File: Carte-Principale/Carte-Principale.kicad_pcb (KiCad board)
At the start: 2 copper layers, 154.6 x 118.1 mm, 115 parts, among them J1 Moteur_Gauche, J10 GPIO, J11 I2C2, J12 GPIO, J13 Encodeur_G, J14 I2C_Sensors, J15 AX12, J16 GPIO, J17 SMD_Conn, J18 PCA9685, J19 GPIO, J2 GND, J3 12VA, J4 5V, J5 Moteur_Droit, J6 UART_Debug, J7 UART, J8 Encodeur_D, J9 SPI3, Q2 BSS138, Q3 BSS138, Q4 BSS138, Q5 BSS138, SW1 Rouge, SW2 Bleu, SW3 Jaune, SW4 Vert, U2 NUCLEOH723ZG, U3 AM26LV32xD, U4 74LVC1G3157, U5 74LVC1G3157, U6 74LVC1G3157, U7 74LVC1G3157

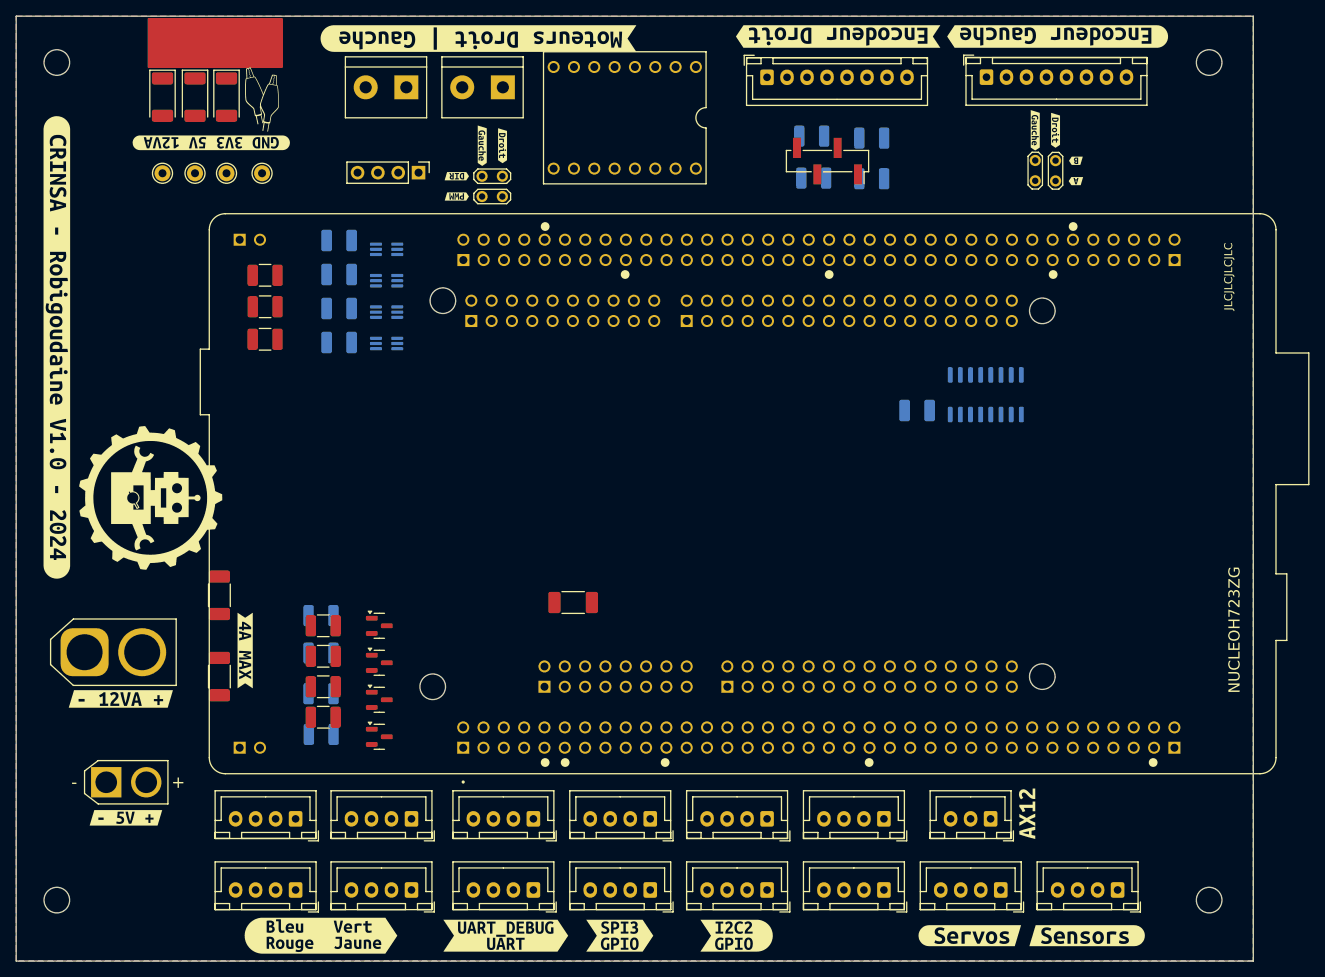
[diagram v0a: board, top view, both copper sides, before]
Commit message: FInal
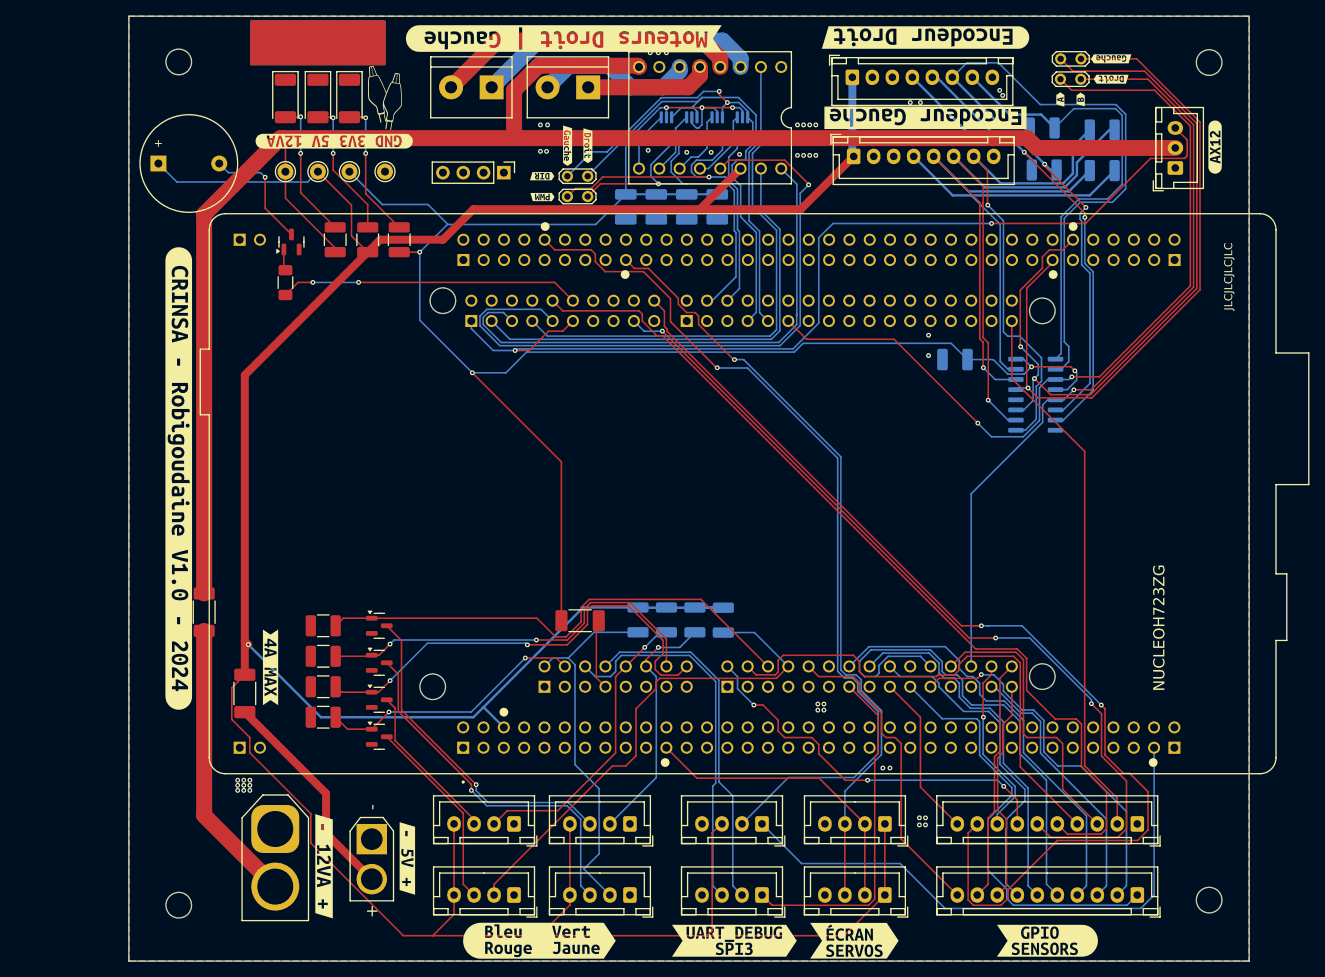
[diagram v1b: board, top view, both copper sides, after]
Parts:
- removed J11: I2C2, Connector_JST:JST_XH_B4B-XH-A_1x04_P2.50mm_Vertical
- removed J12, J16, J19: GPIO, Connector_JST:JST_XH_B4B-XH-A_1x04_P2.50mm_Vertical
- removed J14: I2C_Sensors, Connector_JST:JST_XH_B4B-XH-A_1x04_P2.50mm_Vertical
- removed J17: SMD_Conn, Connector_PinHeader_2.54mm:PinHeader_1x04_P2.54mm_Vertical_SMD_Pin1Right
- removed kibuzzard-11: G***, kibuzzard-66C08EB4
- removed kibuzzard-12: G***, kibuzzard-66C48662
- removed kibuzzard-13: G***, kibuzzard-66C46925
- removed kibuzzard-14: G***, kibuzzard-66C08BB8
- removed kibuzzard-26: G***, kibuzzard-66C091C7
- removed kibuzzard-31: G***, kibuzzard-66C09378
- removed kibuzzard-32: G***, kibuzzard-66C60E06
- removed kibuzzard-33: G***, kibuzzard-66C60E22
- removed kibuzzard-36: G***, kibuzzard-66C09018
- removed kibuzzard-66E9AA77: G***, kibuzzard-66E9AA77
- removed kibuzzard-66F082DD: G***, kibuzzard-66F082DD
- removed kibuzzard-66FEA7C0: G***, kibuzzard-66FEA7C0
- removed kibuzzard-66FEA7DC: G***, kibuzzard-66FEA7DC
- removed kibuzzard-66FEA7EE: G***, kibuzzard-66FEA7EE
- removed kibuzzard-66FEA7FA: G***, kibuzzard-66FEA7FA
- removed kibuzzard-9: G***, kibuzzard-66C092F4
- added BZ1: Buzzer, Buzzer_Beeper:Buzzer_12x9.5RM7.6, F.Cu at (73.7, 47.6)
- added J21: I2C Screen, Connector_JST:JST_XH_B4B-XH-A_1x04_P2.50mm_Vertical, F.Cu at (164.5, 130.2)
- added Q1: BC817, Package_TO_SOT_SMD:SOT-23, F.Cu at (90.3, 57.4)
- added R2: R, Resistor_SMD:R_1206_3216Metric_Pad1.30x1.75mm_HandSolder, F.Cu at (89.5, 62.5)
- added kibuzzard-67547681: G***, kibuzzard-67547681, F.Cu at (145.7, 144.8)
- added kibuzzard-67548783: G***, kibuzzard-67548783, F.Cu at (184.8, 144.8)
- added kibuzzard-67548923: G***, kibuzzard-67548923, F.Cu at (205.7, 45.6)
- added kibuzzard-6754898D: G***, kibuzzard-6754898D, B.Cu at (160.7, 134.6)
- added kibuzzard-675489B9: G***, kibuzzard-675489B9, B.Cu at (160.6, 142.6)
- added kibuzzard-675489F8: G***, kibuzzard-675489F8, B.Cu at (184.8, 143.5)
- added kibuzzard-67548A22: G***, kibuzzard-67548A22, B.Cu at (184.8, 134.0)
- added kibuzzard-67548BCB: G***, kibuzzard-67548BCB, F.Cu at (160.7, 144.8)
- added kibuzzard-6757392E: G***, kibuzzard-6757392E, F.Cu at (121.7, 51.8)
- added kibuzzard-67573990: G***, kibuzzard-67573990, F.Cu at (169.5, 31.9)
- added kibuzzard-675739BC: G***, kibuzzard-675739BC, F.Cu at (169.5, 41.9)
- G1: moved to B.Cu
- J10: value GPIO -> Sensors; footprint Connector_JST:JST_XH_B4B-XH-A_1x04_P2.50mm_Vertical -> Connector_JST:JST_XH_B10B-XH-A_1x10_P2.50mm_Vertical
- J7: value UART -> GPIO; footprint Connector_JST:JST_XH_B4B-XH-A_1x04_P2.50mm_Vertical -> Connector_JST:JST_XH_B10B-XH-A_1x10_P2.50mm_Vertical
- moved kibuzzard-27 90.4 mm to (197.5, 45.8), turned to 0 degrees
- moved J15 84.6 mm to (200.8, 48.2), turned to 90 degrees
- moved J7 75.9 mm to (196.0, 130.2)
- moved G1 74.0 mm to (146.7, 88.9)
- moved J10 60.9 mm to (196.0, 139.1)
- moved R34 52.3 mm to (144.3, 104.7), turned to 90 degrees
- moved U6 52.0 mm to (146.7, 43.2), turned to 90 degrees
- moved C6 50.2 mm to (143.5, 53.0), turned to 90 degrees
- moved U7 47.3 mm to (143.5, 43.2), turned to 90 degrees
- moved R33 46.7 mm to (140.7, 104.7), turned to 90 degrees
- moved C5 45.3 mm to (139.7, 53.0), turned to 90 degrees
- moved R31 44.2 mm to (137.2, 104.7), turned to 90 degrees
- moved U5 42.7 mm to (140.3, 43.2), turned to 90 degrees
- moved C4 40.5 mm to (135.9, 53.0), turned to 90 degrees
- moved R32 39.8 mm to (133.6, 104.7), turned to 90 degrees
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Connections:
- J10 pad 1: /PF8 -> /I2C2_SCL
- J10 pad 2: /PG1 -> /I2C2_SDA
- J10 pad 3: /PG0 -> /PD1
- J10 pad 4: /PD1 -> /PE2
- J7 pad 1: /PC7 -> GND
- J7 pad 2: /PC6 -> /PE0
- J7 pad 3: +5V -> /PF8
- J7 pad 4: GND -> /PD6
- U2 pad CN10_11: /PF6 -> /Encodeur_Droit_A
- U2 pad CN11_11: /Encodeur_Droit_B -> unconnected-(U2A-PF7-PadCN11_11)
- U2 pad CN11_41: /AX12_RX -> unconnected-(U2A-PD5-PadCN11_41)
- U2 pad CN11_6: unconnected-(U2A-5V_EXT-PadCN11_6) -> +5V
- U2 pad CN11_9: /Encodeur_Droit_A -> unconnected-(U2A-PF6-PadCN11_9)
- U2 pad CN12_37: /AX12_RX -> unconnected-(U2B-PA3-PadCN12_37)
- U2 pad CN7_1: /PC6 -> /AX12_RX
- U2 pad CN7_11: /PC7 -> /AX12_RX
- U2 pad CN9_26: /PF7 -> /Encodeur_Droit_B
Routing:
- net +5V: track 0.00 -> 418.8 mm, vias 0 -> 1
- net +3.3V: track 0.00 -> 240.8 mm, vias 0 -> 7
- net +12VA: track 0.00 -> 213.3 mm
- net /PF3: track 0.00 -> 134.4 mm, vias 0 -> 2
- net /AX12_RX: track 0.00 -> 120.8 mm, vias 0 -> 2
- net /PA5: track 0.00 -> 112.2 mm
- net /DEBUG_TX: track 0.00 -> 110.5 mm, vias 0 -> 1
- net /PA4: track 0.00 -> 107.0 mm, vias 0 -> 3
- net /Encodeur_Droit_A: track 0.00 -> 105.1 mm, vias 0 -> 2
- net /Encodeur_Droit_B: track 0.00 -> 98.1 mm, vias 0 -> 1
- net /I2C1_SCL: track 0.00 -> 97.7 mm, vias 0 -> 1
- net /Encodeur_Gauche_A: track 0.00 -> 95.3 mm, vias 0 -> 2
- net /Encodeur_Gauche_B: track 0.00 -> 85.7 mm, vias 0 -> 1
- net /PA15: track 0.00 -> 84.2 mm, vias 0 -> 1
- net /Encodeurs/A+_DROITE: track 0.00 -> 76.1 mm
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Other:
- board size 154.6 x 118.1 mm -> 140 x 118.1 mm
